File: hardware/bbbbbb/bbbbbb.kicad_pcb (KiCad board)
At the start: 2 copper layers, 135.6 x 87.4 mm, 68 parts, among them P1 gondola charge, P2 enable pull up, Q1 Q_NPN_BEC, Q2 Q_NPN_BEC, Q3 BS170, U1 xbee, U2 LTV-827, U3 LTV-827, U4 LTV-827, U5 drv2250, U6 drv2250, U9 LM358

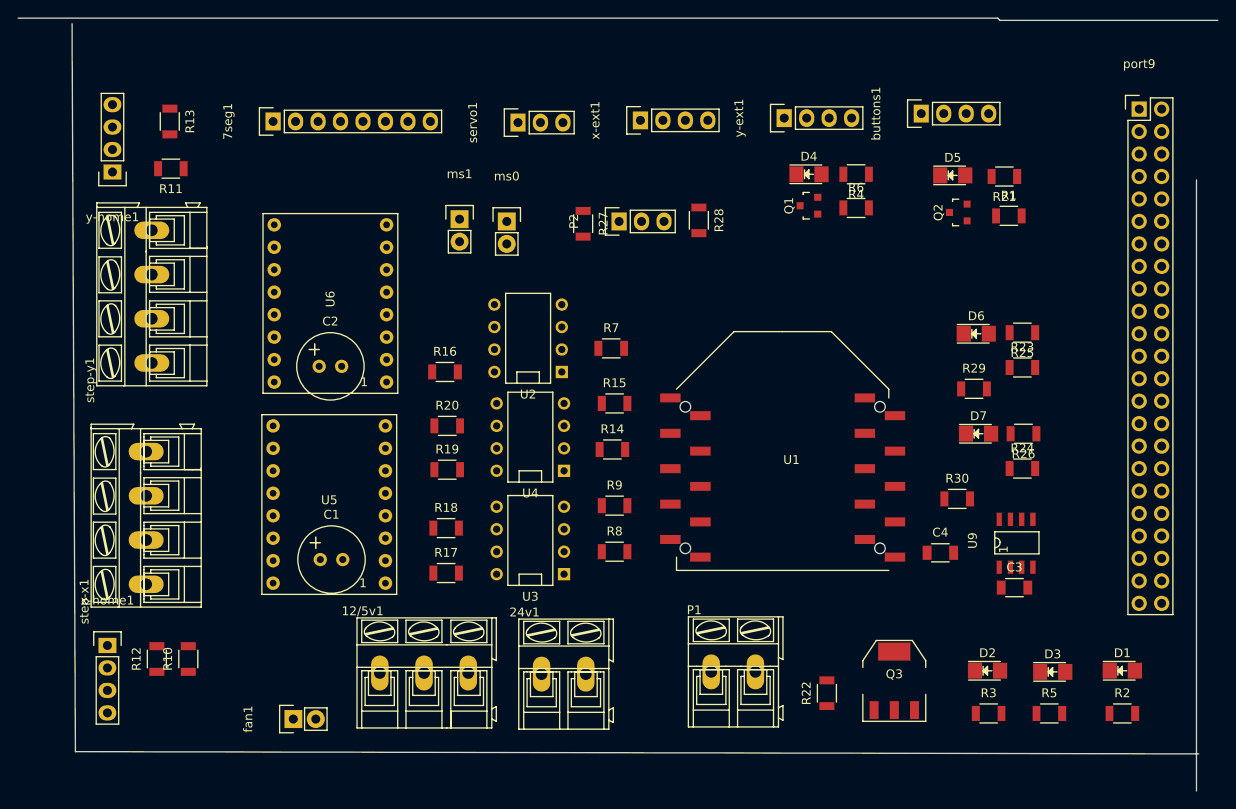
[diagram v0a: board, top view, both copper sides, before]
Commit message: gondola charge
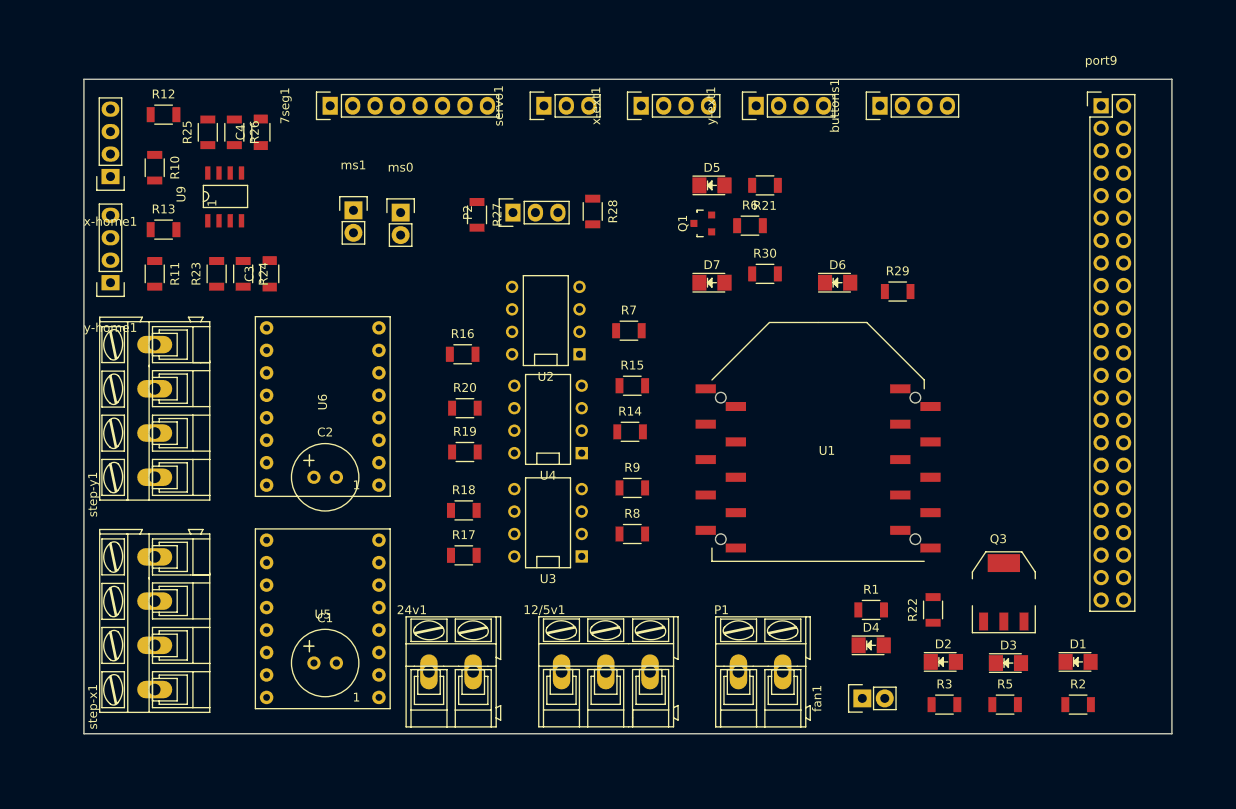
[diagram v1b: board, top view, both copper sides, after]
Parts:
- removed Q2: Q_NPN_BEC, Housings_SOT-23_SOT-143_TSOT-6:SOT-23
- removed R4: R, Resistors_SMD:R_1206
- moved U9 97.7 mm to (163.0, 98.0)
- moved R26 95.5 mm to (163.0, 90.0), turned to 270 degrees
- moved R25 94.8 mm to (160.0, 90.0), turned to 90 degrees
- moved R23 91.7 mm to (161.0, 106.0), turned to 90 degrees
- moved C3 91.4 mm to (167.0, 106.0), turned to 90 degrees
- moved R24 90.8 mm to (164.0, 106.0), turned to 270 degrees
- moved C4 90.3 mm to (166.0, 90.0), turned to 90 degrees
- moved fan1 64.4 mm to (234.0, 154.0)
- moved R12 61.5 mm to (155.0, 88.0), turned to 0 degrees
- moved R10 55.7 mm to (154.0, 94.0), turned to 270 degrees
- moved D4 53.7 mm to (235.0, 148.0)
- moved x-home1 53.0 mm to (149.0, 95.0), turned to 180 degrees
- moved R1 47.2 mm to (235.0, 144.0)
- moved D7 34.6 mm to (217.0, 107.0)
- moved R30 33.5 mm to (223.0, 106.0)
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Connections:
- P1 pad 1: +24V -> +5V
- P1 pad 2: Net-(P1-Pad2) -> Net-(D4-Pad1)
- Q1 pad 2: Earth -> (no net)
- Q3 pad 1: Net-(P1-Pad2) -> Net-(D4-Pad1)
- R1 pad 1: Net-(Q2-Pad1) -> +5V
- R1 pad 2: gondola-charge -> Net-(D4-Pad2)
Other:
- board size 135.6 x 87.4 mm -> 123 x 74 mm
